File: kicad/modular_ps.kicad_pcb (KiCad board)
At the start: 2 copper layers, 21 parts, among them J1 PJ-102AH, U1 LM7812_TO220, U2 LM7912_TO220

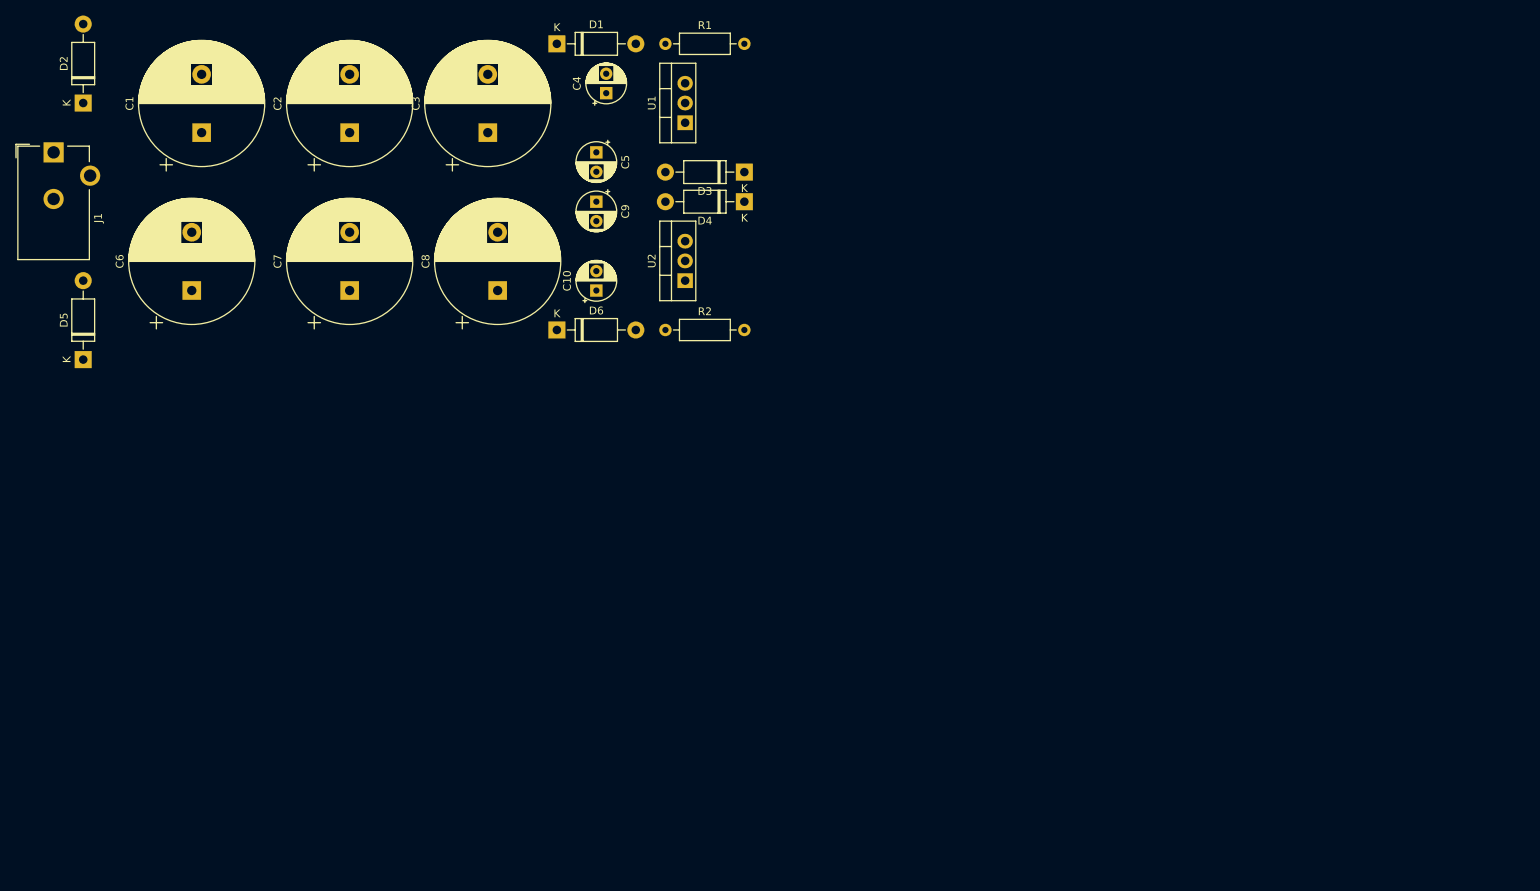
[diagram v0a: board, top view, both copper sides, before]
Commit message: commit for V1
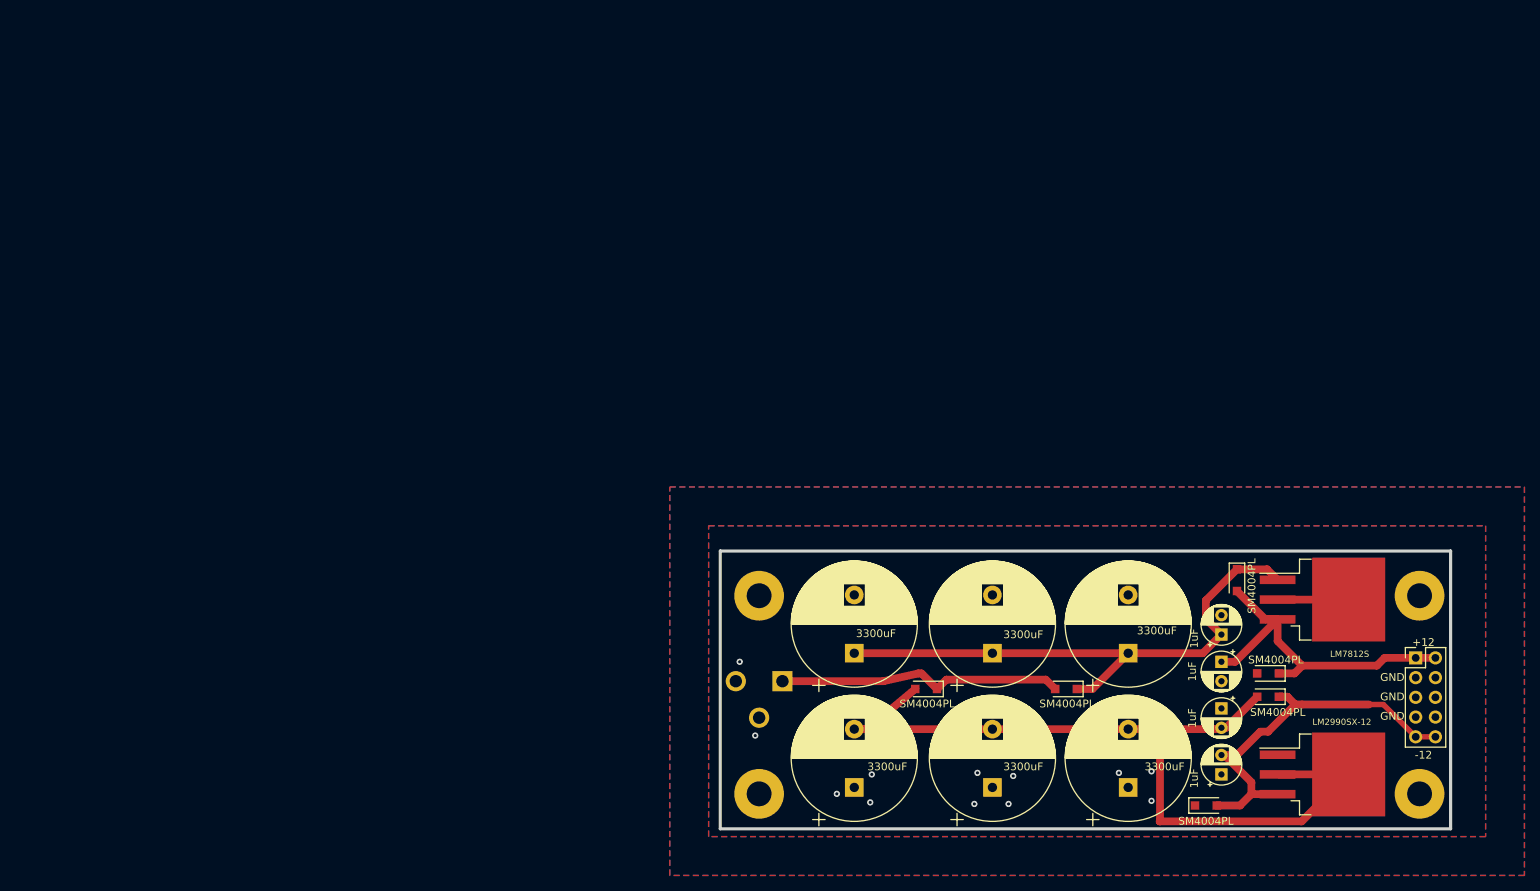
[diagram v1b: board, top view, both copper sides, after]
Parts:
- removed D1, D2, D3, D4, D5, D6: 1N4004, Diode_THT:D_DO-41_SOD81_P10.16mm_Horizontal
- removed R1, R2: 2.4K, Resistor_THT:R_Axial_DIN0207_L6.3mm_D2.5mm_P10.16mm_Horizontal
- added J2: Conn_02x05_Counter_Clockwise, Connector_PinHeader_2.54mm:PinHeader_2x05_P2.54mm_Vertical, F.Cu at (188.0, 93.0)
- added REF**: MountingHole_3.2mm_M3_Pad, MountingHole:MountingHole_3.2mm_M3_Pad, F.Cu at (188.5, 85.0)
- added REF**: MountingHole_3.2mm_M3_Pad, MountingHole:MountingHole_3.2mm_M3_Pad, F.Cu at (188.5, 110.5)
- added REF**: MountingHole_3.2mm_M3_Pad, MountingHole:MountingHole_3.2mm_M3_Pad, F.Cu at (103.5, 110.5)
- added REF**: MountingHole_3.2mm_M3_Pad, MountingHole:MountingHole_3.2mm_M3_Pad, F.Cu at (103.5, 85.0)
- added SM4004PL: SM4004PL-TP, Diode_SMD:D_SOD-123F, F.Cu at (161.0, 112.0)
- added SM4004PL: SM4004PL-TP, Diode_SMD:D_SOD-123F, F.Cu at (125.0, 97.0)
- added SM4004PL: SM4004PL-TP, Diode_SMD:D_SOD-123F, F.Cu at (169.0, 98.0)
- added SM4004PL: SM4004PL-TP, Diode_SMD:D_SOD-123F, F.Cu at (169.0, 95.0)
- added SM4004PL: SM4004PL-TP, Diode_SMD:D_SOD-123F, F.Cu at (143.0, 97.0)
- added SM4004PL: SM4004PL-TP, Diode_SMD:D_SOD-123F, F.Cu at (165.0, 83.0)
- U1: value LM7812_TO220 -> LM7812S; footprint Package_TO_SOT_THT:TO-220-3_Vertical -> Package_TO_SOT_SMD:TO-263-3_TabPin2
- U2: value LM7912_TO220 -> LM2990SX-12; footprint Package_TO_SOT_THT:TO-220-3_Vertical -> Package_TO_SOT_SMD:TO-263-3_TabPin2
- moved J1 115.9 mm to (106.5, 96.0), turned to 270 degrees
- moved C1 107.4 mm to (115.7, 92.4)
- moved C6 106.6 mm to (115.7, 109.7)
- moved C2 106.5 mm to (133.5, 92.4)
- moved C3 106.2 mm to (151.0, 92.4)
- moved C4 105.5 mm to (163.0, 90.0)
- moved C7 104.6 mm to (133.5, 109.7)
- moved C5 103.8 mm to (163.0, 93.5)
- moved U2 103.8 mm to (176.0, 108.0), turned to 0 degrees
- moved C9 103.6 mm to (163.0, 99.5)
- moved C8 103.3 mm to (151.0, 109.7)
- moved U1 102.4 mm to (176.0, 85.5), turned to 0 degrees
- moved C10 101.7 mm to (163.0, 108.0)
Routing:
- net Net-(C6-Pad2): track 0.00 -> 112.6 mm
- net Net-(C1-Pad1): track 0.00 -> 75.9 mm
- net -12V: track 0.00 -> 49.7 mm
- net +12V: track 0.00 -> 45.2 mm
- net Net-(D2-Pad2): track 0.00 -> 37.0 mm
- net GND: track 0.00 -> 9.15 mm, vias 0 -> 21
- added copper zone on B.Cu, net GND
- added copper zone on F.Cu, net GND
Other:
- board outline added: 94 x 35.8 mm
- net class Default: clearance 0.2 -> 0.1524; trace_width 0.25 -> 0.1524; via_dia 0.8 -> 0.6858; via_drill 0.4 -> 0.3302
- rule pad_to_mask_clearance: 0.05 -> 0.0508
- rule trace_clearance: 0.2 -> 0.1524
- rule trace_min: 0.2 -> 0.1524
- rule via_min_drill: 0.3 -> 0.254
- rule via_min_size: 0.4 -> 0.508
- board text added: "+12"
- board text added: "-12"
- board text added: "GND"
- board text added: "MFOS Wall Wart To Bipolar Power Supply"
- board text added: "Sam Zeter October 2020"
